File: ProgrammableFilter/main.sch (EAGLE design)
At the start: 42 parts, among them IC1 TL074P, IC2 LM324N, IC3 MAX261, IC4 4053N, IC5 4053N, IC7 TL072P, U2 ADG509AKR

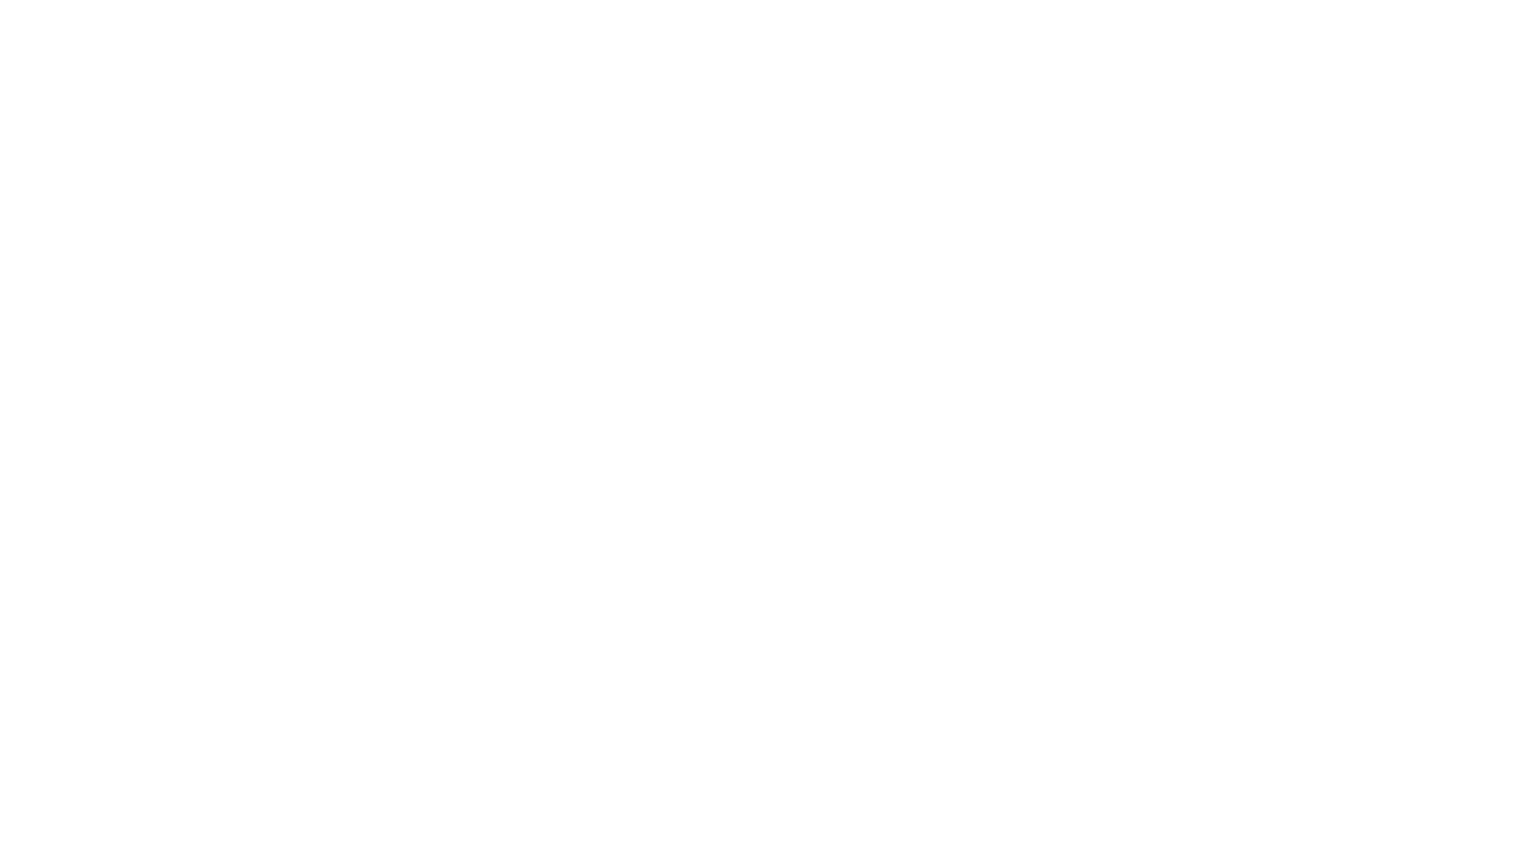
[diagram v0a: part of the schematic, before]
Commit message: updated eagle epf
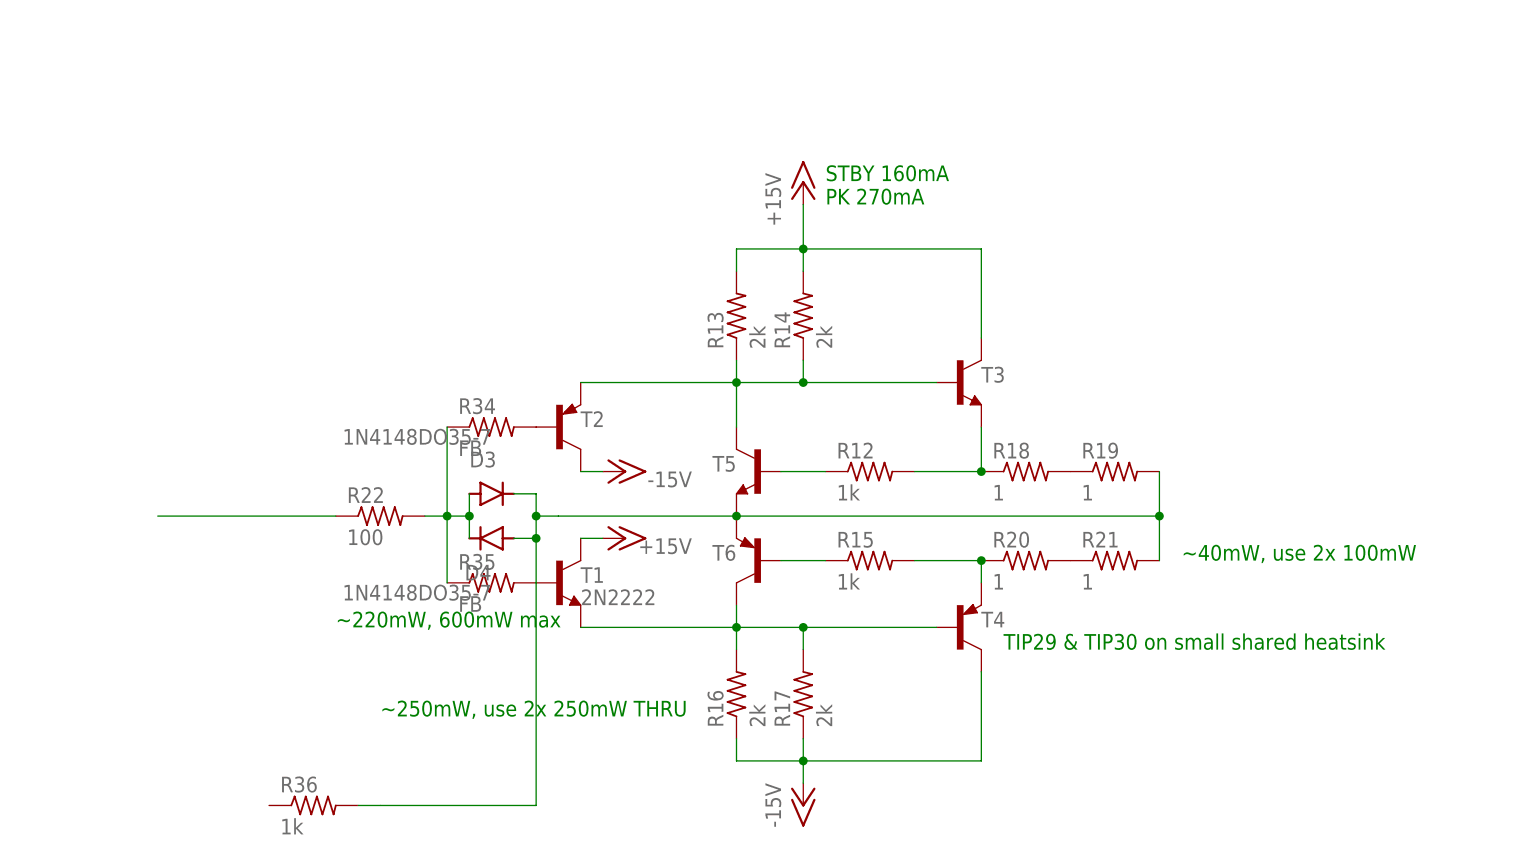
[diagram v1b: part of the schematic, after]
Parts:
- added D3, D4: 1N4148DO35-7, diode:1N4148DO35-7
- added R12, R15, R36: 1k, resistor:R-US_0207/7
- added R13, R14, R16, R17: 2k, resistor:R-US_0207/2V
- added R18, R19, R20, R21: 1, resistor:R-US_R0805
- added R22: 100, resistor:R-US_0207/7
- added R34, R35: FB, resistor:R-US_0207/7
- added T1: 2N2222, adafruit:2N2222
- added T2: (no value), DC_LOAD_AU:BC557A-PNP-TO92-EBC
- added T3: (no value), DC_LOAD_AU:-NPN-TO220V
- added T4: (no value), DC_LOAD_AU:-PNP-TO220V
- added T5: (no value), transistor:MMBT3904LT1-NPN-SOT23-BEC
- added T6: (no value), transistor:MMBT3906LT1-PNP-SOT23-BEC
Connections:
- new net +15V: R13.2, R14.2, T1.C, T3.C
- new net -15V: R16.1, R17.1, T2.C, T4.C
- new net N$24: D3.C, D4.A, R19.2, R21.2, R36.2, T5.E, T6.E
- new net N$25: R16.2, R17.2, T1.E, T4.B, T6.C
- new net N$26: R15.1, T6.B
- new net N$27: R15.2, R20.1, T4.E
- new net N$28: R12.1, T5.B
- new net N$29: R12.2, R18.1, T3.E
- new net N$30: R13.1, R14.1, T2.E, T3.B, T5.C
- new net N$32: R18.2, R19.1
- new net N$33: R20.2, R21.1
- new net N$34: R22.1
- new net N$36: R35.2, T1.B
- new net N$48: D3.A, D4.C, R22.2, R34.1, R35.1
- new net N$49: R34.2, T2.B
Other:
- note added: "STBY 160mA PK 270mA"
- note added: "TIP29 & TIP30 on small shared heatsink"
- note added: "~220mW, 600mW max"
- note added: "~250mW, use 2x 250mW THRU"
- note added: "~40mW, use 2x 100mW"
